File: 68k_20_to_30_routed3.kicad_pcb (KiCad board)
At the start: 4 copper layers, 86 x 78.5 mm, 6 parts, among them U1 68030, U2 68020

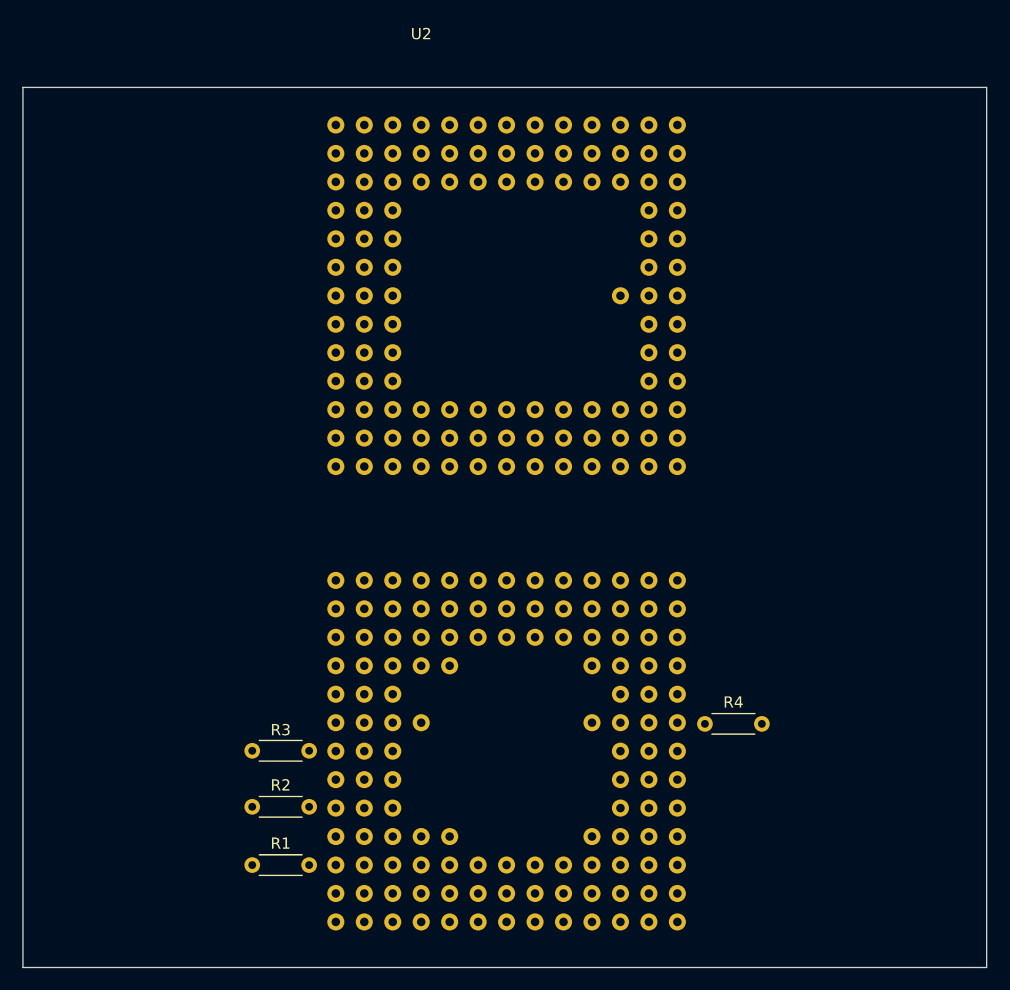
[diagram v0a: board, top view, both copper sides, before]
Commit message: Adding current state of routing.
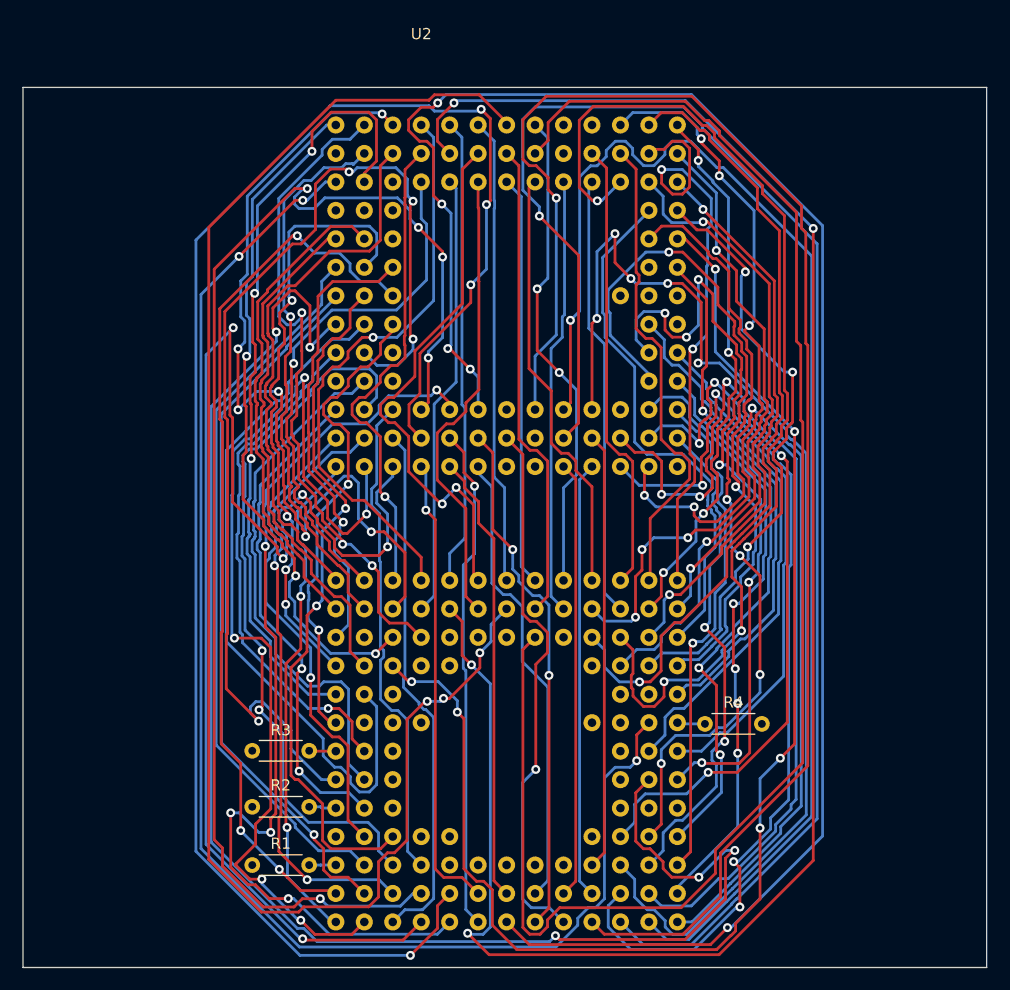
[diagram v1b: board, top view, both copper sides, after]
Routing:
- net /A27: track 0.00 -> 166.2 mm, vias 0 -> 4
- net /D19: track 0.00 -> 159.4 mm, vias 0 -> 5
- net /D24: track 0.00 -> 148.3 mm, vias 0 -> 4
- net /A18: track 0.00 -> 139.4 mm
- net /A22: track 0.00 -> 138.7 mm, vias 0 -> 3
- net /D13: track 0.00 -> 137.4 mm, vias 0 -> 1
- net /D15: track 0.00 -> 136.5 mm, vias 0 -> 1
- net Net-(U1-CDIS): track 0.00 -> 135.3 mm, vias 0 -> 5
- net /RESET: track 0.00 -> 125.6 mm, vias 0 -> 3
- net /OCS: track 0.00 -> 120.7 mm, vias 0 -> 6
- net /D11: track 0.00 -> 120.2 mm, vias 0 -> 1
- net /D25: track 0.00 -> 119.9 mm, vias 0 -> 5
- net /D27: track 0.00 -> 118.3 mm, vias 0 -> 5
- net /D7: track 0.00 -> 104.2 mm, vias 0 -> 5
- net /BERR: track 0.00 -> 96.8 mm, vias 0 -> 4
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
